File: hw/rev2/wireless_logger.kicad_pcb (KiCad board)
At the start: 4 copper layers, 30 x 50 mm, 153 parts, among them J1 FCI 10118194, J2 CONN_2, J3 SSD1306_SER, J4 SWD_10PIN, J5 CONN_5, J6 CONN_6X2, Q1 2N7002P, Q2 2N7002P, U1 MT29FXX01A, U10 CC2541, U11 STM32F40X_BGA176, U2 MAG3110, U3 MMA8452Q, U4 LPS331AP, U5 L3GD20, U6 MCP111T-315, U7 BQ24095, U8 TPS62698, U9 CC1101, X1 FA-128 26.0000MF10Z-W3, X2 9HT10-32.768KBZF-T, X3 FA-128 32.0000MF20X-K3, X4 XRCGB25M000F0L00R0, X5 9HT10-32.768KBZF-T

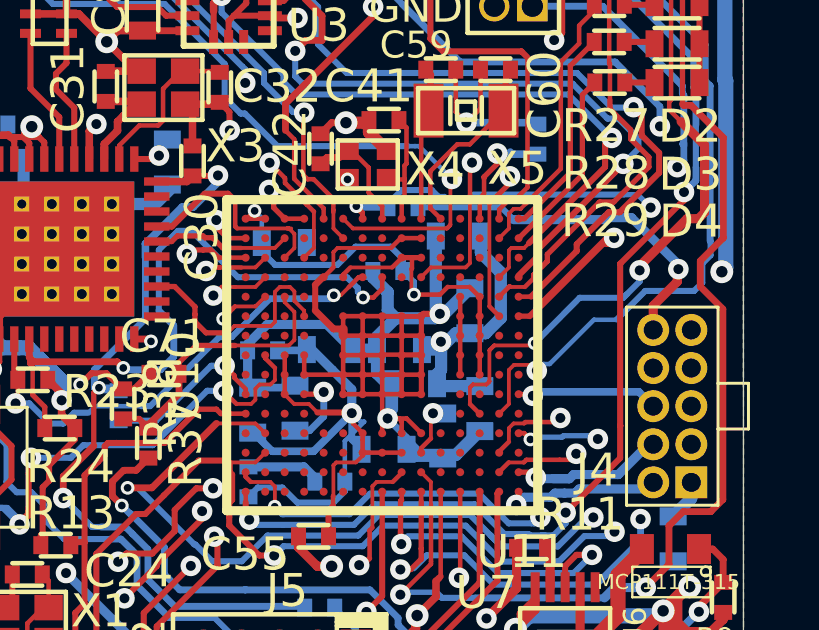
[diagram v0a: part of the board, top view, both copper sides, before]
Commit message: Finished more small connections
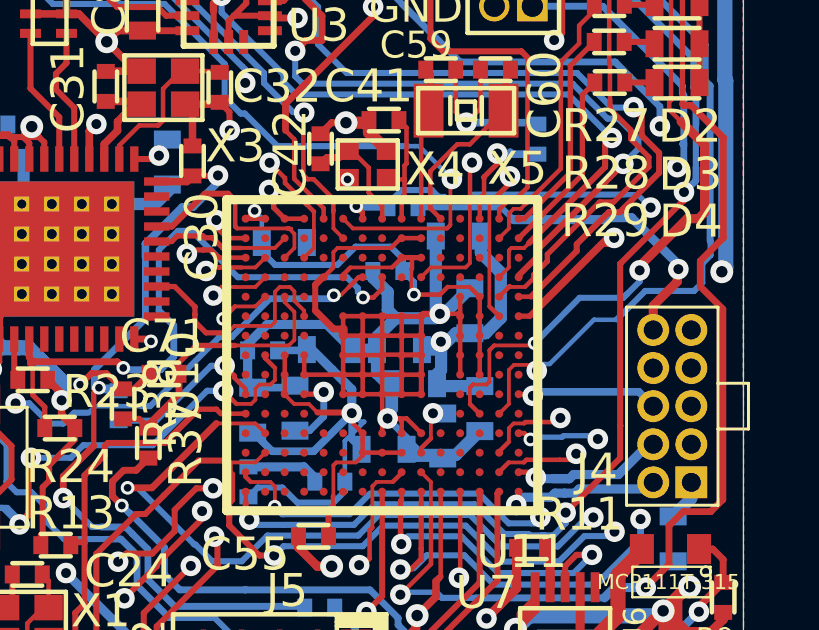
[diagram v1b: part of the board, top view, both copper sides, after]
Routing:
- net GND: track 288.0 -> 288.7 mm
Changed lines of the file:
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@@
   (general
     (links 490)
-    (no_connects 1)
-    (area 169.994999 109.994999 200.005001 160.005001)
+    (no_connects 0)
+    (area 162.356596 104.978178 209.633231 164.898333)
     (thickness 1.6)
     (drawings 18)
-    (tracks 3234)
+    (tracks 3236)
     (zones 0)
     (modules 153)
@@
   (layers
     (15 F.Cu signal)
-    (2 Inner2.Cu mixed)
-    (1 GND_PLANE mixed)
+    (2 Inner2.Cu mixed hide)
+    (1 GND_PLANE mixed hide)
     (0 B.Cu signal)
     (16 B.Adhes user hide)
@@
   )
   (setup
-    (last_trace_width 0.1778)
+    (last_trace_width 0.1524)
     (user_trace_width 0.127)
     (user_trace_width 0.1524)
@@
     (pad_to_mask_clearance 0)
     (aux_axis_origin 0 0)
-    (visible_elements FFFF7F8F)
+    (visible_elements FFFF7FAF)
     (pcbplotparams
       (layerselection 284196871)
@@
   (segment (start 189.63641 131.419884) (end 189.63641 122.14859) (width 0.2032) (layer Inner2.Cu) (net 60))
   (segment (start 189.63641 122.14859) (end 190.08852 121.69648) (width 0.2032) (layer Inner2.Cu) (net 60))
-  (segment (start 188.07684 121.97842) (end 188.07684 122.51055) (width 0.3048) (layer F.Cu) (net 61) (status 400000))
-  (segment (start 188.22924 122.83059) (end 188.22924 123.2782) (width 0.3048) (layer B.Cu) (net 61) (status 800000))
+  (segment (start 188.07684 121.97842) (end 188.07684 122.51055) (width 0.3048) (layer F.Cu) (net 61))
+  (segment (start 188.22924 122.83059) (end 188.22924 123.2782) (width 0.3048) (layer B.Cu) (net 61))
   (segment (start 187.99302 122.59437) (end 188.22924 122.83059) (width 0.3048) (layer B.Cu) (net 61))
   (via (at 187.99302 122.59437) (size 0.4572) (drill 0.254) (layers F.Cu B.Cu) (net 61))
@@
   (segment (start 185.28919 124.48536) (end 185.29173 124.48282) (width 0.254) (layer F.Cu) (net 61))
   (segment (start 182.29326 124.7902) (end 183.09336 124.7902) (width 0.2286) (layer B.Cu) (net 61) (status 40030))
+  (segment (start 189.88024 141.69644) (end 190.47652 141.69644) (width 0.1524) (layer F.Cu) (net 62) (status 800000))
+  (segment (start 190.47652 141.69644) (end 190.5566 141.77652) (width 0.1524) (layer F.Cu) (net 62) (status C00000))
   (segment (start 189.57544 124.78328) (end 190.76092 124.78328) (width 0.254) (layer B.Cu) (net 62))
   (via (at 190.9826 124.5616) (size 0.4572) (drill 0.254) (layers F.Cu B.Cu) (net 62))
@@
   (segment (start 185.03138 141.63421) (end 185.03138 142.56639) (width 0.127) (layer F.Cu) (net 112))
   (segment (start 184.7066 141.30943) (end 185.03138 141.63421) (width 0.127) (layer F.Cu) (net 112))
-  (segment (start 188.07684 123.9774) (end 188.07684 124.50699) (width 0.254) (layer F.Cu) (net 113) (status 400000))
+  (segment (start 188.07684 123.9774) (end 188.07684 124.50699) (width 0.254) (layer F.Cu) (net 113))
   (segment (start 188.46927 125.67285) (end 188.05398 126.08814) (width 0.1778) (layer F.Cu) (net 113))
   (segment (start 188.46927 124.89942) (end 188.46927 125.67285) (width 0.1778) (layer F.Cu) (net 113))
